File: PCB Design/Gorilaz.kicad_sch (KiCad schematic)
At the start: 57 parts, among them J1 Conn_01x13, J2 Conn_01x13, J3 Conn_01x13, J4 Conn_01x13, J5 HRO_TYPE-C-31-M-14, J5 Thermistor, J6 Battery, J6 Thermistor, J7 Conn_01x13, J8 Conn_01x13, J9 Battery, J9 TC2030_SWD, Q2 2N7002, SW1 PWR, SW4 RST, U1 SRV05-4, U10 MAX17048, U3 BQ24075, U4 DW01A, U5 FS8205, U8 nRF52840_moko_mk08

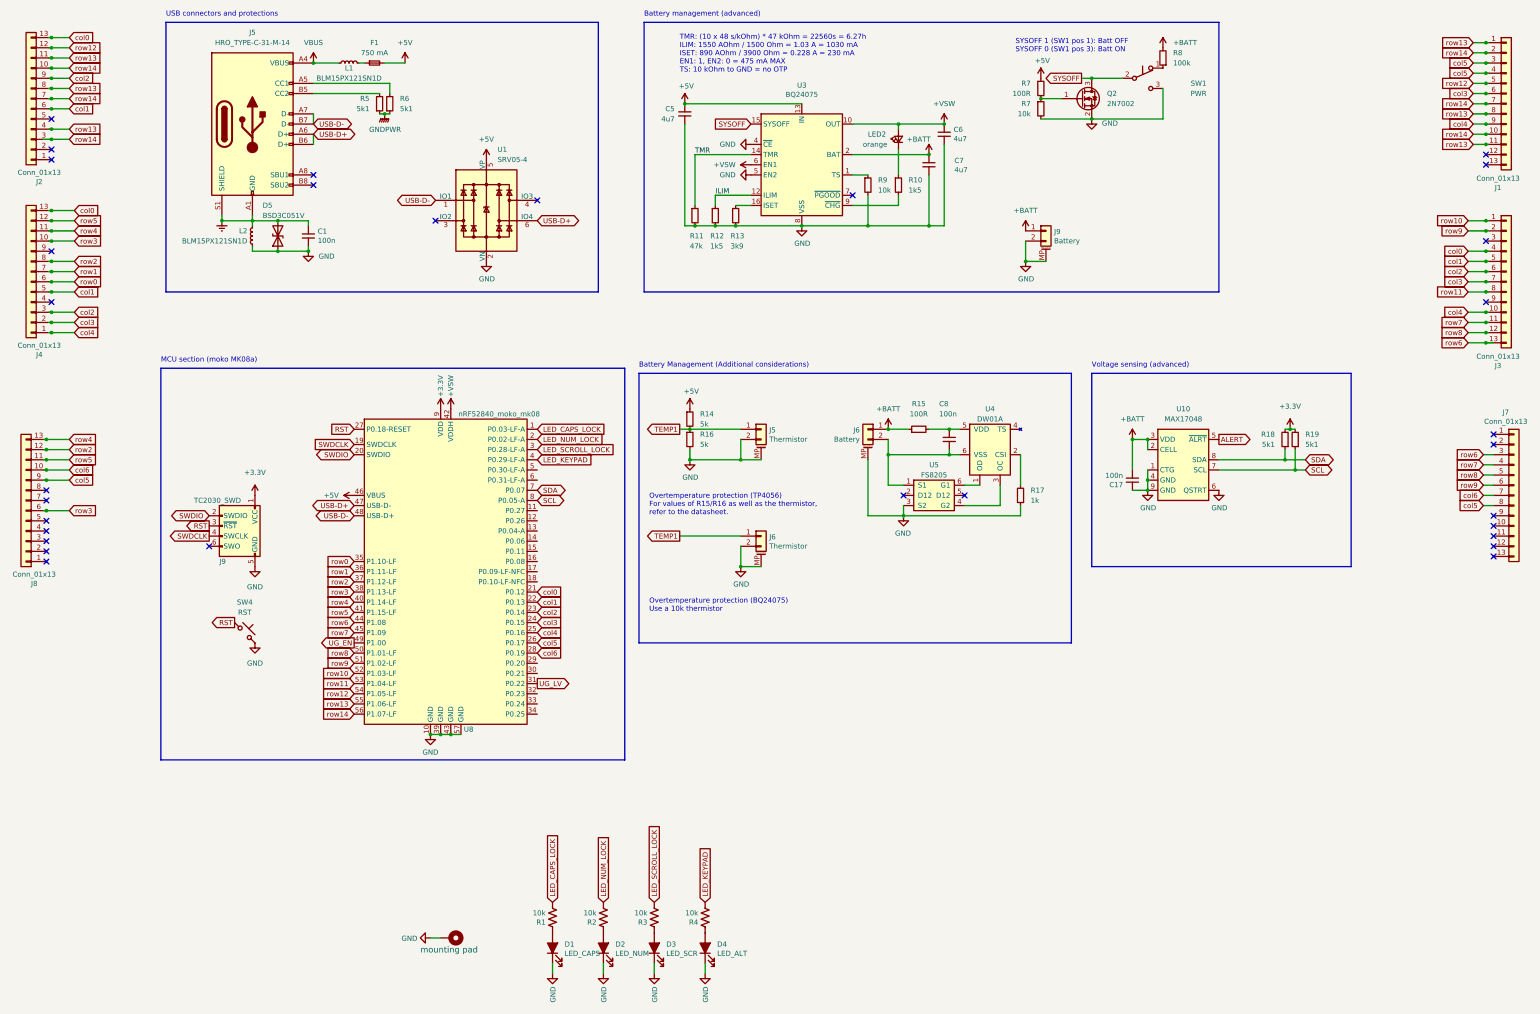
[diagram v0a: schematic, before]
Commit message: schema update
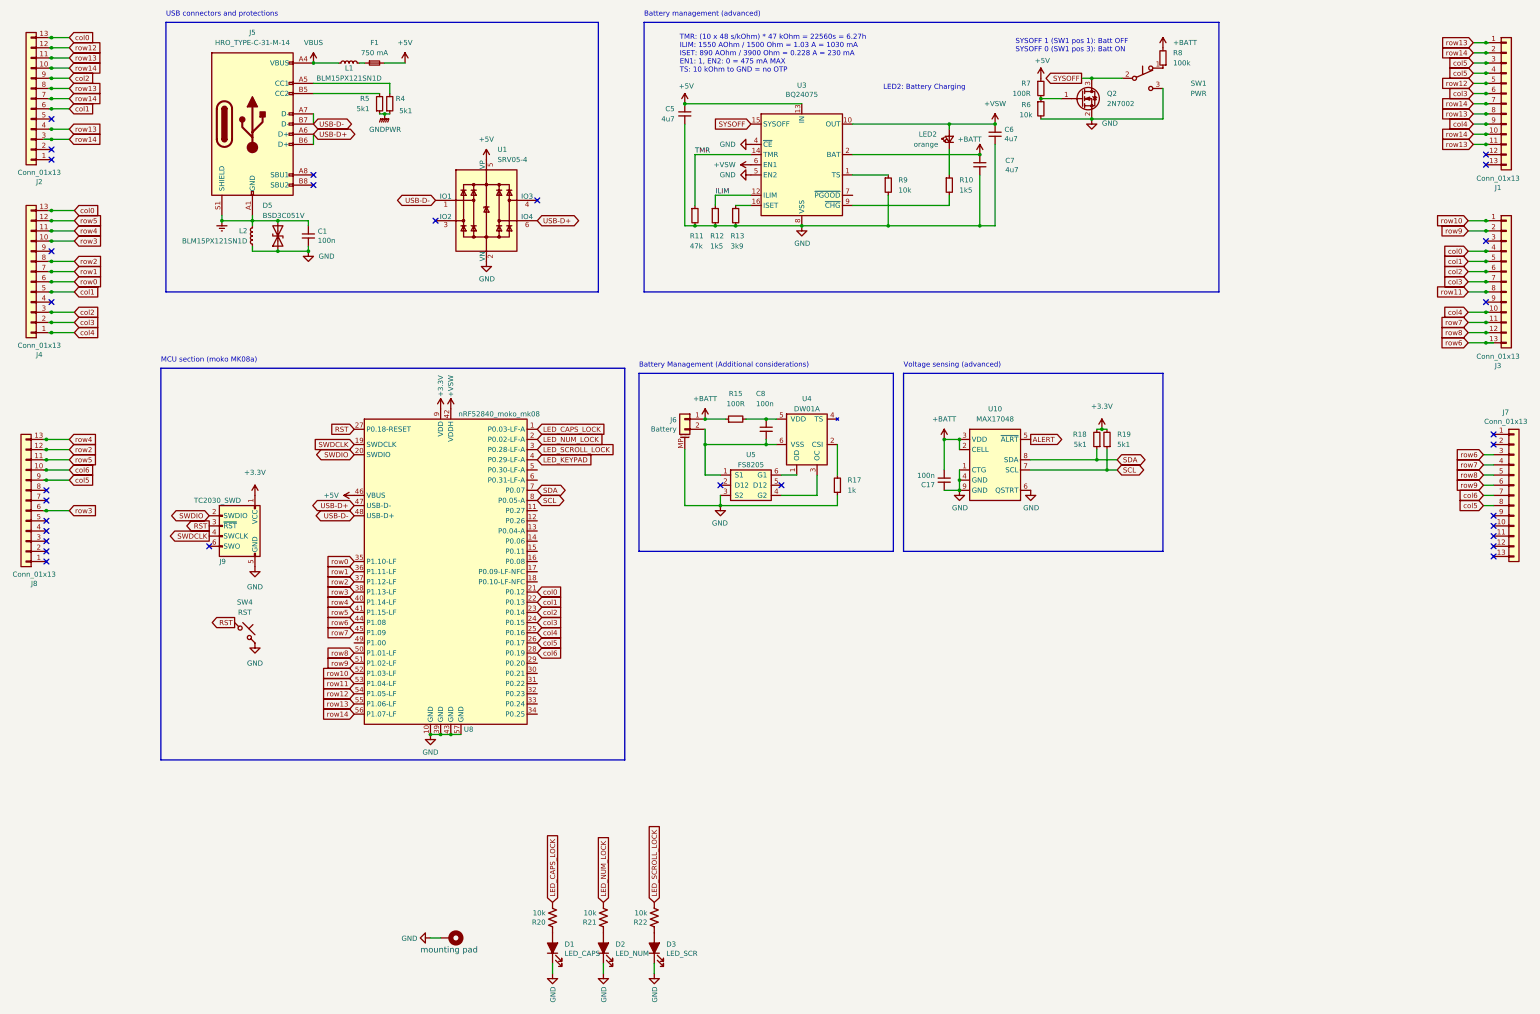
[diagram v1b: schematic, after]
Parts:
- removed D4: LED_ALT, LED_SMD:LED_1206_3216Metric, symbol kicad_port-rescue:LED_ALT-Device
- removed J5, J6: Thermistor, Connector_JST:JST_PH_S2B-PH-K_1x02_P2.00mm_Horizontal, symbol Connector_Generic_MountingPin:Conn_01x02_MountingPin
- removed J9: Battery, PCM_marbastlib-various:Molex_Pico-EZmate_78171-0002_1x02-1MP_P1.20mm_Vertical, symbol Connector_Generic_MountingPin:Conn_01x02_MountingPin
- removed R14, R16: 5k, Resistor_SMD:R_0402_1005Metric, symbol Device:R_Small
- removed R4: 10k, Resistor_SMD:R_0805_2012Metric, symbol kicad_port-rescue:R_US-Device
- J1, J2, J7, J8: footprint kinesisMod_board_connectors:Molex_0039532135 -> Local:Molex_0039532135
- J3: footprint kinesisMod_board_connectors:Molex_039532134 -> Local:Molex_0039532135
- J4: footprint kinesisMod_board_connectors:Molex_039532134 -> Molex_0039532135
- J6: footprint PCM_marbastlib-various:Molex_Pico-EZmate_78171-0002_1x02-1MP_P1.20mm_Vertical -> Local:Molex_Pico-EZmate_78171-0002_1x02-1MP_P1.20mm_Vertical
- J9: footprint PCM_marbastlib-various:CON_TC2030_outlined -> Local:CON_TC2030_outlined
- SW1: footprint PCM_marbastlib-various:SW_MSK12C02-HB -> Mastarlib:SW_MSK12C02-HB
- SW4: footprint PCM_marbastlib-various:SW_SPST_SKQG_WithStem -> Button_Switch_SMD:SW_SPST_SKQG_WithStem
- U10: footprint Package_DFN_QFN:DFN-8-1EP_2x2mm_P0.5mm_EP0.7x1.3mm -> Local:DFN-8-1EP_2x2mm_P0.5mm_EP0.7x1.3mm
- U8: footprint PCM_marbastlib-various:nRF52840_moko_mk08 -> Mastarlib:nRF52840_moko_mk08
- renumbered R1 to R20, R2 to R21, R3 to R22, R6 to R4, R7 to R6
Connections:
- net UG_EN: no longer names the net of U8.49 (P1.00)
- net UG_LV: no longer names the net of U8.31 (P0.22)
- no-connect marks 31 -> 30
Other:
- note added: "LED2: Battery Charging"
- note removed: "Overtemperature protection (BQ24075) Use a 10k thermistor"
- note removed: "Overtemperature protection (TP4056) For values of R15/R16 as well as the thermistor, refer to the datasheet."
- moved on the sheet: C17, C6, C7, C8, J6, LED2, R10, R15, R17, R18, R19, R9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

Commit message: v0
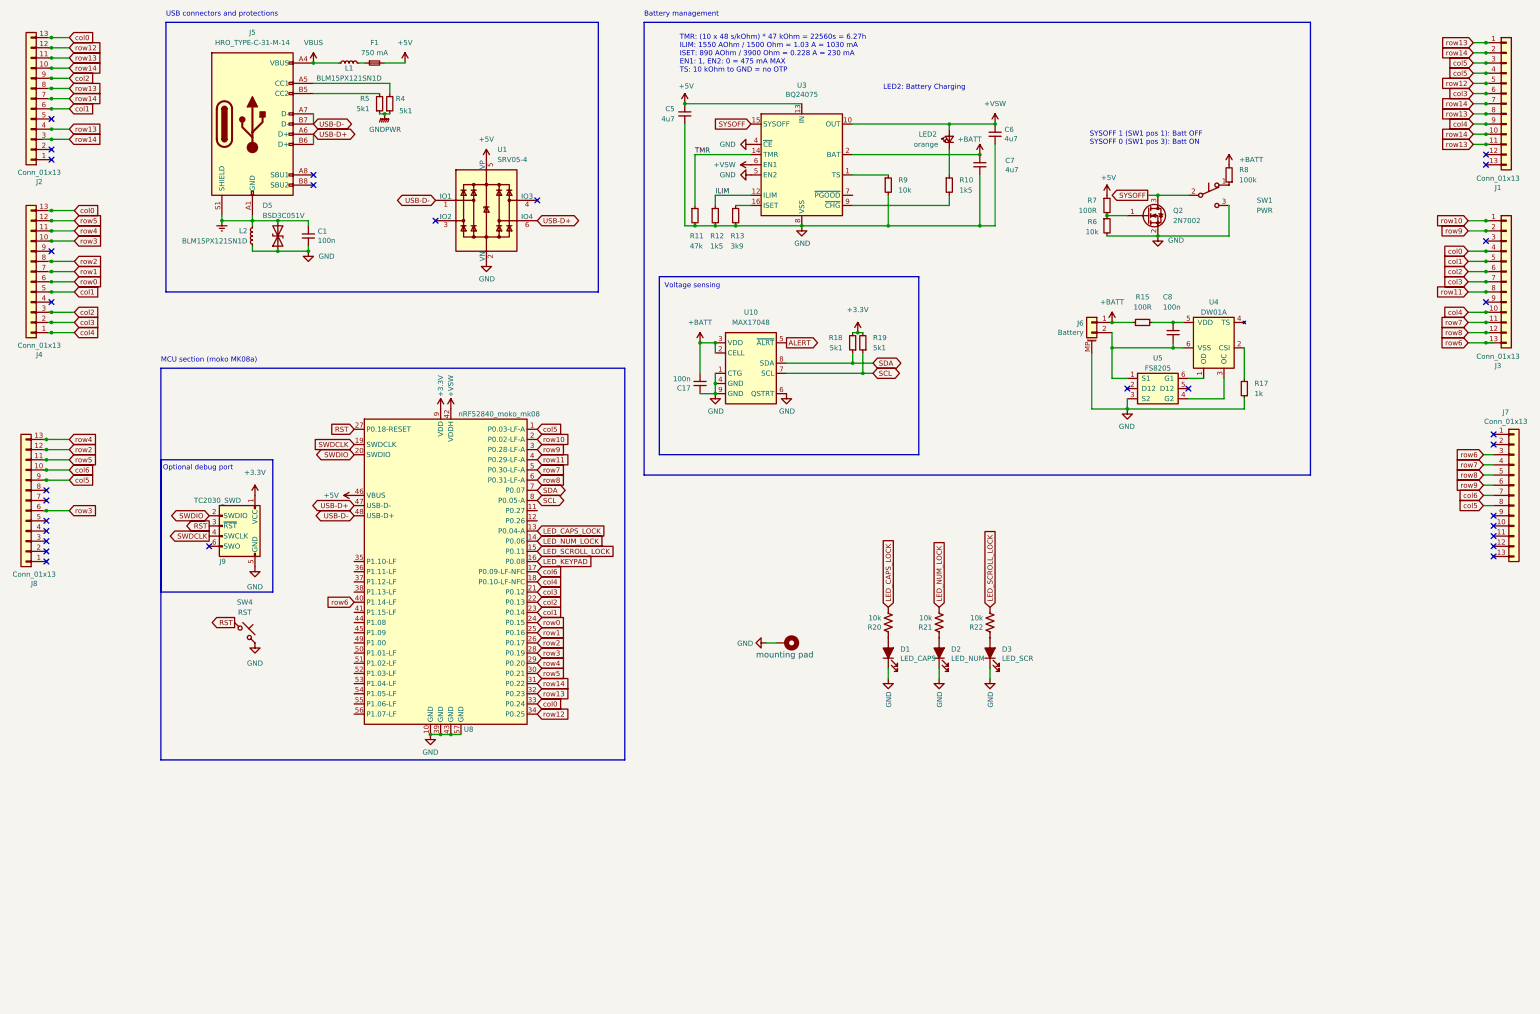
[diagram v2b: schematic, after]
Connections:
- net LED_CAPS_LOCK: now also U8.13 (P0.04-A); no longer U8.1 (P0.03-LF-A)
- net LED_KEYPAD: now also U8.16 (P0.08); no longer U8.4 (P0.29-LF-A)
- net LED_NUM_LOCK: now also U8.14 (P0.06); no longer U8.2 (P0.02-LF-A)
- net LED_SCROLL_LOCK: now also U8.15 (P0.11); no longer U8.3 (P0.28-LF-A)
- net col0: now also U8.33 (P0.24); no longer U8.21 (P0.12)
- net col1: now also U8.23 (P0.14); no longer U8.22 (P0.13)
- net col2: now also U8.22 (P0.13); no longer U8.23 (P0.14)
- net col3: now also U8.21 (P0.12); no longer U8.24 (P0.15)
- net col4: now also U8.18 (P0.10-LF-NFC); no longer U8.25 (P0.16)
- net col5: now also U8.1 (P0.03-LF-A); no longer U8.26 (P0.17)
- net col6: now also U8.17 (P0.09-LF-NFC); no longer U8.28 (P0.19)
- net row0: now also U8.24 (P0.15); no longer U8.35 (P1.10-LF)
- net row1: now also U8.25 (P0.16); no longer U8.36 (P1.11-LF)
- net row10: now also U8.2 (P0.02-LF-A); no longer U8.52 (P1.03-LF)
- net row11: now also U8.4 (P0.29-LF-A); no longer U8.53 (P1.04-LF)
- net row12: now also U8.34 (P0.25); no longer U8.54 (P1.05-LF)
- net row13: now also U8.32 (P0.23); no longer U8.55 (P1.06-LF)
- net row14: now also U8.31 (P0.22); no longer U8.56 (P1.07-LF)
- net row2: now also U8.26 (P0.17); no longer U8.37 (P1.12-LF)
- net row3: now also U8.28 (P0.19); no longer U8.38 (P1.13-LF)
- net row4: now also U8.29 (P0.20); no longer U8.40 (P1.14-LF)
- net row5: now also U8.30 (P0.21); no longer U8.41 (P1.15-LF)
- net row6: now also U8.40 (P1.14-LF); no longer U8.44 (P1.08)
- net row7: now also U8.5 (P0.30-LF-A); no longer U8.45 (P1.09)
- net row8: now also U8.6 (P0.31-LF-A); no longer U8.50 (P1.01-LF)
- net row9: now also U8.3 (P0.28-LF-A); no longer U8.51 (P1.02-LF)
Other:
- note added: "Battery management"
- note added: "Optional debug port"
- note added: "Voltage sensing"
- note removed: "Battery Management (Additional considerations)"
- note removed: "Battery management (advanced)"
- note removed: "Voltage sensing (advanced)"
- moved on the sheet: C17, C8, D1, D2, D3, J6, Q2, R15, R17, R18, R19, R20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
